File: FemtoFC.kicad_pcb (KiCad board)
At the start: 4 copper layers, 17.5 x 50.1 mm, 64 parts, among them J1 Power in, J2 Conn_01x02_Male, J3 Micro_SD_Card, J4 Pyro 2, J5 Pyro 1, P1 USB_C_Plug_USB2.0, Q1 FDS9926A, Q2 FDS4953, Q3 NDT3055L, U1 USBLC6-2SC6, U2 3.3v REG, U3 ATSAMD21G18A-M, U4 W25Q128JVS, U5 LSM6DS3, U6 BMP280, Y1 Crystal

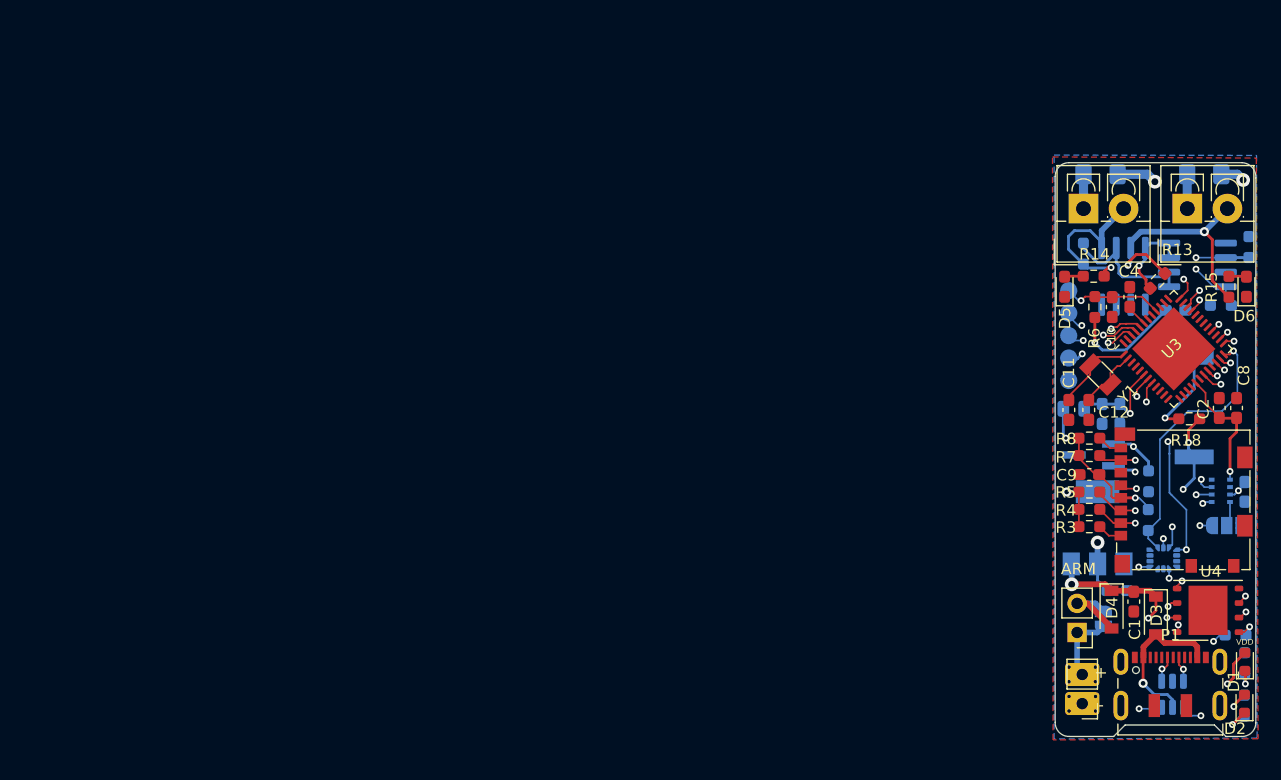
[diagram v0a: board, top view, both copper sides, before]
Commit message: V3
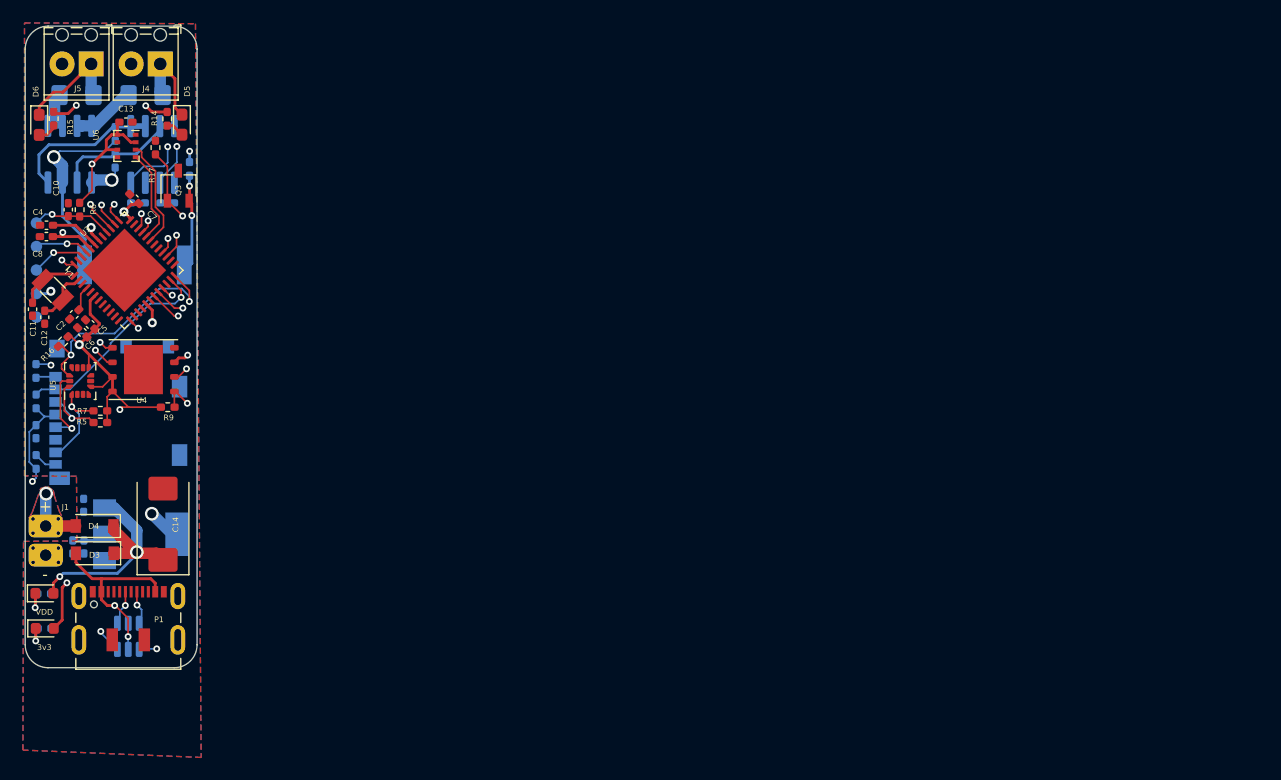
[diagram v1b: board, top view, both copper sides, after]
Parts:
- removed D1, D2: G, LED_SMD:LED_0603_1608Metric
- removed FB1: FerriteBead_Small, Resistor_SMD:R_0805_2012Metric
- removed J2: Conn_01x02_Male, Connector_PinHeader_2.54mm:PinHeader_1x02_P2.54mm_Vertical
- removed JP1: SolderJumper_2_Open, Jumper:SolderJumper-2_P1.3mm_Open_RoundedPad1.0x1.5mm
- removed JP2: SolderJumper_3_Open, Jumper:SolderJumper-3_P1.3mm_Open_RoundedPad1.0x1.5mm
- removed TP1, TP2, TP3, TP4, TP5: TestPoint, TestPoint:TestPoint_Pad_D1.0mm
- added 3v3: G, LED_SMD:LED_0603_1608Metric, F.Cu at (81.7, 90.6)
- added 3v3: TestPoint, TestPoint:TestPoint_Pad_D1.0mm, B.Cu at (81.0, 61.3)
- added C14: 220uF 16V, Capacitor_Tantalum_SMD:CP_EIA-7343-31_Kemet-D, F.Cu at (92.0, 81.5)
- added C15: 1uF, Capacitor_SMD:C_0402_1005Metric_Pad0.74x0.62mm_HandSolder, B.Cu at (84.1, 83.5)
- added GND: TestPoint, TestPoint:TestPoint_Pad_D1.0mm, B.Cu at (81.0, 63.4)
- added RST: TestPoint, TestPoint:TestPoint_Pad_D1.0mm, B.Cu at (81.0, 55.2)
- added SWCLK: TestPoint, TestPoint:TestPoint_Pad_D1.0mm, B.Cu at (81.0, 57.2)
- added SWDIO: TestPoint, TestPoint:TestPoint_Pad_D1.0mm, B.Cu at (81.0, 59.3)
- added VDD: G, LED_SMD:LED_0603_1608Metric, F.Cu at (81.7, 87.5)
- C1: value 100nF -> 10uf; footprint Capacitor_SMD:C_0603_1608Metric_Pad1.08x0.95mm_HandSolder -> Capacitor_SMD:C_0402_1005Metric_Pad0.74x0.62mm_HandSolder; moved to B.Cu
- C10, C11, C12, C3, C8: footprint Capacitor_SMD:C_0603_1608Metric_Pad1.08x0.95mm_HandSolder -> Capacitor_SMD:C_0402_1005Metric_Pad0.74x0.62mm_HandSolder
- C13, C5, C6, C7: footprint Capacitor_SMD:C_0603_1608Metric_Pad1.08x0.95mm_HandSolder -> Capacitor_SMD:C_0402_1005Metric_Pad0.74x0.62mm_HandSolder; moved to F.Cu
- C2: value 10uF -> 1uF; footprint Capacitor_SMD:C_0603_1608Metric_Pad1.08x0.95mm_HandSolder -> Capacitor_SMD:C_0402_1005Metric_Pad0.74x0.62mm_HandSolder
- C4: value 100nF -> 1uF; footprint Capacitor_SMD:C_0603_1608Metric_Pad1.08x0.95mm_HandSolder -> Capacitor_SMD:C_0402_1005Metric_Pad0.74x0.62mm_HandSolder
- C9: value 100nF -> 10uF; footprint Capacitor_SMD:C_0603_1608Metric_Pad1.08x0.95mm_HandSolder -> Capacitor_SMD:C_0402_1005Metric_Pad0.74x0.62mm_HandSolder; moved to B.Cu
- J3: moved to B.Cu
- J4: footprint TerminalBlock_4Ucon:TerminalBlock_4Ucon_1x02_P3.50mm_Vertical -> TerminalBlock_Phoenix:TerminalBlock_Phoenix_MPT-0,5-2-2.54_1x02_P2.54mm_Horizontal
- J5: value Pyro 1 -> Pyro 2; footprint TerminalBlock_4Ucon:TerminalBlock_4Ucon_1x02_P3.50mm_Vertical -> TerminalBlock_Phoenix:TerminalBlock_Phoenix_MPT-0,5-2-2.54_1x02_P2.54mm_Horizontal
- Q3: footprint Package_TO_SOT_SMD:TSOT-23_HandSoldering -> Package_TO_SOT_SMD:TSOT-23; moved to F.Cu
- R1, R10, R11, R12, R14, R15, R2, R5, R6, R7: footprint Resistor_SMD:R_0603_1608Metric_Pad0.98x0.95mm_HandSolder -> Resistor_SMD:R_0402_1005Metric_Pad0.72x0.64mm_HandSolder
- R13, R18, R3, R4, R8: footprint Resistor_SMD:R_0603_1608Metric_Pad0.98x0.95mm_HandSolder -> Resistor_SMD:R_0402_1005Metric_Pad0.72x0.64mm_HandSolder; moved to B.Cu
- R16, R17, R9: footprint Resistor_SMD:R_0603_1608Metric_Pad0.98x0.95mm_HandSolder -> Resistor_SMD:R_0402_1005Metric_Pad0.72x0.64mm_HandSolder; moved to F.Cu
- U5, U6: moved to F.Cu
- moved D6 106.3 mm to (81.2, 46.6), turned to -90 degrees
- moved R1 105.0 mm to (81.7, 87.5), turned to 0 degrees
- moved C8 105.0 mm to (81.8, 56.4), turned to 180 degrees
- moved R2 104.9 mm to (81.7, 90.6), turned to 0 degrees
- moved R15 103.6 mm to (82.5, 46.1), turned to -90 degrees
- moved C13 102.9 mm to (88.8, 46.4), turned to 0 degrees
- moved C2 100.3 mm to (84.3, 63.2), turned to -135 degrees
- moved U6 100.2 mm to (88.8, 48.5)
- moved F2 98.7 mm to (84.5, 44.0), turned to 0 degrees
- moved J5 96.5 mm to (85.8, 41.3), turned to 180 degrees
- moved R16 96.0 mm to (83.3, 65.5), turned to -135 degrees
- moved U5 95.8 mm to (84.8, 69.0), turned to 90 degrees
- moved R9 95.3 mm to (92.4, 71.3)
- moved U4 95.3 mm to (90.3, 68.0)
- moved R10 94.9 mm to (89.8, 53.4), turned to 180 degrees
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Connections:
- C13 pad 1: VDDIN -> VDDANA
- C2 pad 1: GNDANA -> AREF
- C2 pad 2: VDDIN -> GNDANA
- C3 pad 1: VDDIN -> VDDANA
- C7 pad 1: VDDIN -> VDDANA
- C8 pad 1: VDDIN -> VDDANA
- C9 pad 1: VDDIN -> VDDANA
- D5 pad 1: GNDANA -> Net-(D5-Pad1)
- D6 pad 1: GNDANA -> Net-(D6-Pad1)
- F1 pad 1: +BATT -> Net-(F1-Pad1)
- F1 pad 2: Net-(F1-Pad2) -> Net-(D5-Pad1)
- F2 pad 1: +BATT -> Net-(F2-Pad1)
- F2 pad 2: Net-(F2-Pad2) -> Net-(D6-Pad1)
- J1 pad 2: Net-(J1-Pad2) -> +BATT
- J3 pad 4: VDDIN -> VDDANA
- J4 pad 1: Net-(F1-Pad2) -> Net-(D5-Pad1)
- J4 pad 2: Net-(J4-Pad2) -> GNDANA
- J5 pad 1: Net-(F2-Pad2) -> Net-(D6-Pad1)
- J5 pad 2: Net-(J5-Pad2) -> GNDANA
- P1 pad S1: GNDANA -> unconnected-(P1-PadS1)
- Q1 pad 2: P1_EN -> P2_EN
- Q1 pad 4: P2_EN -> P1_EN
- Q1 pad 5: Net-(Q1-Pad5) -> Net-(Q2-Pad4)
- Q1 pad 6: Net-(Q1-Pad5) -> Net-(Q2-Pad4)
- Q1 pad 7: Net-(Q1-Pad7) -> Net-(Q2-Pad2)
- Q1 pad 8: Net-(Q1-Pad7) -> Net-(Q2-Pad2)
- Q2 pad 1: Net-(J4-Pad2) -> +BATT
- Q2 pad 2: Net-(Q1-Pad5) -> Net-(Q2-Pad2)
- Q2 pad 3: Net-(J5-Pad2) -> +BATT
- Q2 pad 4: Net-(Q1-Pad7) -> Net-(Q2-Pad4)
- Q2 pad 5: GNDANA -> Net-(F2-Pad1)
- Q2 pad 6: GNDANA -> Net-(F2-Pad1)
- Q2 pad 7: GNDANA -> Net-(F1-Pad1)
- Q2 pad 8: GNDANA -> Net-(F1-Pad1)
- R12 pad 1: Net-(Q1-Pad5) -> Net-(Q2-Pad2)
- R12 pad 2: Net-(J4-Pad2) -> +BATT
- R13 pad 1: Net-(Q1-Pad7) -> Net-(Q2-Pad4)
- R13 pad 2: Net-(J5-Pad2) -> +BATT
- R14 pad 1: Net-(J4-Pad2) -> +BATT
- R15 pad 1: Net-(J5-Pad2) -> +BATT
- R16 pad 1: VDDIN -> VDDANA
- R3 pad 2: VDDIN -> VDDANA
- R4 pad 2: VDDIN -> VDDANA
- R5 pad 2: VDDIN -> VDDANA
- R6 pad 1: VDDIN -> VDDANA
- R7 pad 2: VDDIN -> VDDANA
- R8 pad 2: VDDIN -> VDDANA
- R9 pad 1: VDDIN -> VDDANA
- U2 pad 2: VDDIN -> VDDANA
- U3 pad 10: unconnected-(U3-Pad10) -> A4
- U3 pad 13: unconnected-(U3-Pad13) -> Buzzer
- U3 pad 14: unconnected-(U3-Pad14) -> D3
- U3 pad 17: VDDIN -> VDDANA
- U3 pad 19: P2_EN -> MOSI
- U3 pad 20: P1_EN -> SCK
- U3 pad 21: unconnected-(U3-Pad21) -> MISO
- U3 pad 22: SPI_CS_FLASH -> unconnected-(U3-Pad22)
- U3 pad 25: MOSI -> unconnected-(U3-Pad25)
- U3 pad 26: SCK -> unconnected-(U3-Pad26)
- U3 pad 27: unconnected-(U3-Pad27) -> P1_EN
- U3 pad 28: MISO -> P2_EN
- U3 pad 3: unconnected-(U3-Pad3) -> A0
- U3 pad 31: unconnected-(U3-Pad31) -> SDA
- U3 pad 32: unconnected-(U3-Pad32) -> SCL
- U3 pad 36: VDDIN -> VDDANA
- U3 pad 37: unconnected-(U3-Pad37) -> FLASH_MOSI
- U3 pad 38: unconnected-(U3-Pad38) -> FLASH_SCK
- U3 pad 39: unconnected-(U3-Pad39) -> SPI_CS_FLASH
- U3 pad 4: unconnected-(U3-Pad4) -> AREF
- U3 pad 44: VDDIN -> VDDANA
- U3 pad 48: unconnected-(U3-Pad48) -> FLASH_MISO
- U3 pad 7: SDA -> unconnected-(U3-Pad7)
- U3 pad 8: SCL -> unconnected-(U3-Pad8)
- U3 pad 9: unconnected-(U3-Pad9) -> A3
- U4 pad 2: MISO -> FLASH_MISO
- U4 pad 3: VDDIN -> VDDANA
- U4 pad 5: MOSI -> FLASH_MOSI
- U4 pad 6: SCK -> FLASH_SCK
- U4 pad 7: VDDIN -> VDDANA
- U4 pad 8: VDDIN -> VDDANA
- U5 pad 5: VDDIN -> VDDANA
- U5 pad 8: VDDIN -> VDDANA
- U6 pad 2: VDDIN -> VDDANA
- U6 pad 5: Net-(JP2-Pad2) -> GNDANA
- U6 pad 6: VDDIN -> VDDANA
- U6 pad 8: VDDIN -> VDDANA
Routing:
- net VDDIN: track 65.0 -> 0.00 mm, vias 19 -> 0
- net VDDANA: track 8.42 -> 69.9 mm, vias 1 -> 12
- net MOSI: track 78.1 -> 23.4 mm, vias 4 -> 2
- net SCK: track 65.6 -> 24.4 mm, vias 4 -> 2
- net FLASH_MISO: track 0.00 -> 31.8 mm, vias 0 -> 2
- net Net-(J5-Pad2): track 22.8 -> 0.00 mm, vias 2 -> 0
- net SCL: track 29.0 -> 8.22 mm, vias 2 -> 0
- net FLASH_SCK: track 0.00 -> 17.4 mm, vias 0 -> 2
- net MISO: track 40.9 -> 23.9 mm, vias 5 -> 2
- net SDA: track 26.3 -> 9.59 mm, vias 2 -> 0
- net FLASH_MOSI: track 0.00 -> 15.7 mm, vias 0 -> 2
- net Net-(J4-Pad2): track 15.0 -> 0.00 mm, vias 1 -> 0
- net Buzzer: track 4.50 -> 18.8 mm, vias 1 -> 2
- net SPI_CS_FLASH: track 29.1 -> 42.5 mm
- net Net-(Q2-Pad4): track 0.00 -> 13.1 mm
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- added copper zone on B.Cu, net +BATT
- added copper zone on F.Cu, net +BATT
- added copper zone on In2.Cu, net GNDANA
- added copper zone on In1.Cu, net VDDANA
- removed copper zone on In2.Cu, net VDDIN
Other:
- board size 17.5 x 50.1 mm -> 15 x 56 mm
- board text removed: "0x76"
- board text removed: "0x77"
- board text removed: "ARM"
- board text removed: "CLK"
- board text removed: "GND"
- board text removed: "RST"
- board text removed: "SWDIO"
- board text removed: "VDD"
